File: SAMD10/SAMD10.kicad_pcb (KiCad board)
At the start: 2 copper layers, 18 x 34 mm, 15 parts, among them J0 SWD_PGM, J1 GPIO_A, J2 GPIO_B, J3 Battery, SW1 SW_Push, U1 ATSAMD10C14A-SS, U2 AP7333-33SRG-7

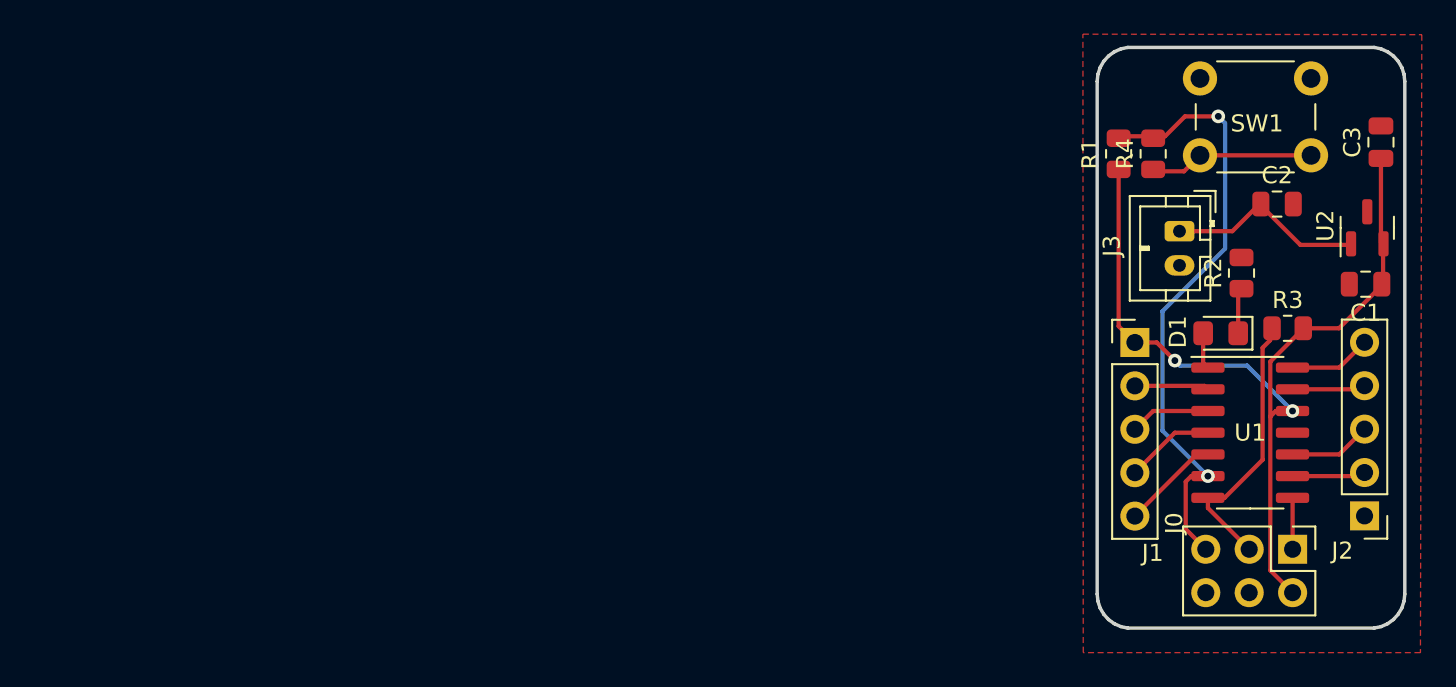
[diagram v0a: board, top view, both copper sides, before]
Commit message: update schematics
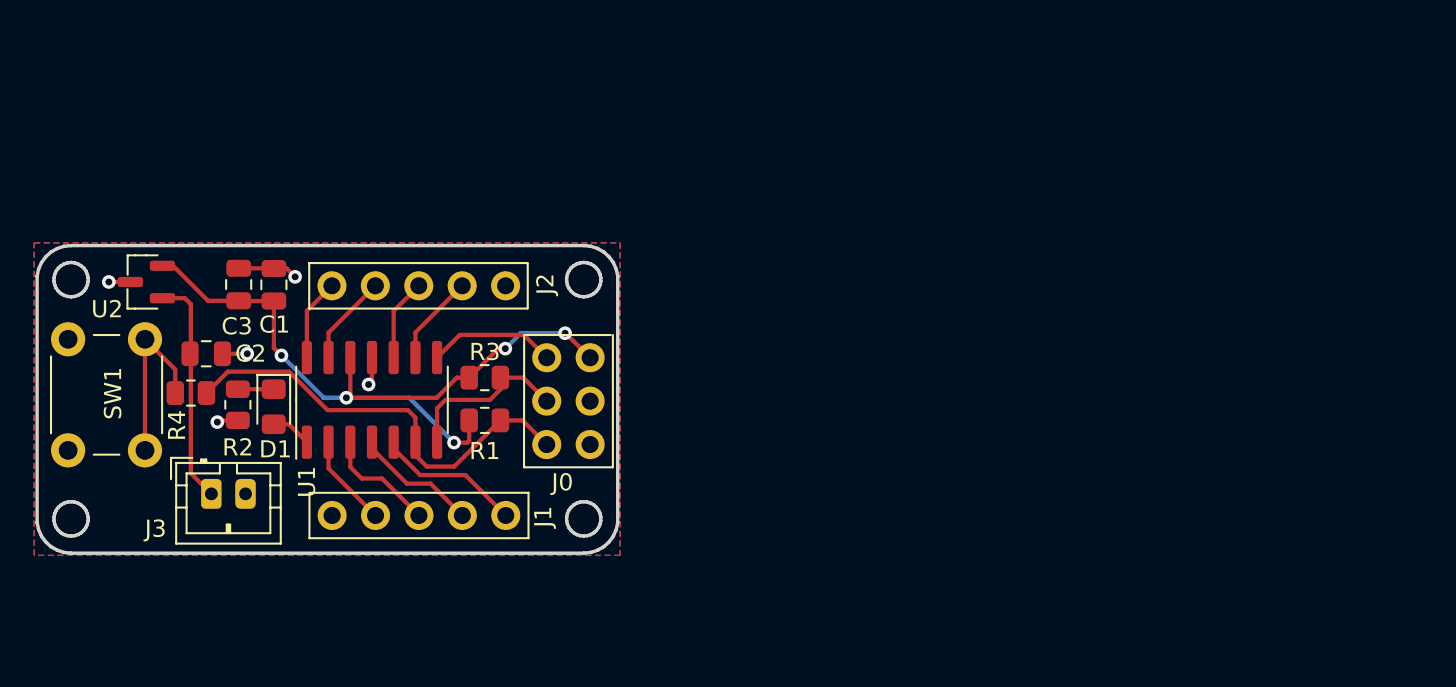
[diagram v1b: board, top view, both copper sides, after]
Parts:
- moved U2 71.5 mm to (135.6, 95.0), turned to 180 degrees
- moved SW1 69.1 mm to (135.5, 98.4), turned to -90 degrees
- moved C3 67.4 mm to (141.0, 95.2)
- moved C1 63.9 mm to (143.1, 95.2), turned to 90 degrees
- moved C2 63.3 mm to (139.1, 99.2)
- moved R2 59.2 mm to (140.9, 102.2), turned to -90 degrees
- moved J3 58.7 mm to (139.4, 107.4), turned to 0 degrees
- moved R4 58.0 mm to (138.2, 101.5), turned to 0 degrees
- moved D1 55.6 mm to (143.1, 102.3), turned to -90 degrees
- moved J2 52.0 mm to (156.6, 95.2), turned to -90 degrees
- moved U1 51.4 mm to (148.8, 101.9), turned to 90 degrees
- moved J1 48.1 mm to (146.5, 108.7), turned to 90 degrees
- moved R3 47.1 mm to (155.4, 100.6), turned to 180 degrees
- moved J0 45.1 mm to (159.0, 99.4), turned to 0 degrees
- moved R1 40.2 mm to (155.4, 103.1), turned to 0 degrees
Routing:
- net RESET: track 36.0 -> 25.7 mm, vias 2 -> 0
- net GND: track 0.00 -> 9.12 mm, vias 0 -> 5
- net +3V3: track 52.6 -> 43.9 mm, vias 2 -> 5
- net SWCLK: track 16.0 -> 10.7 mm
- net SWDIO: track 3.01 -> 7.52 mm
- net GPIO_4: track 5.77 -> 8.55 mm
- net GPIO_3: track 5.24 -> 7.28 mm
- net GPIO_2: track 4.72 -> 6.65 mm
- net +BATT: track 11.7 -> 13.4 mm
- net GPIO_6: track 4.30 -> 5.63 mm
- net GPIO_8: track 4.30 -> 5.63 mm
- net GPIO_1: track 4.36 -> 5.43 mm
- net Net-(R4-Pad1): track 9.63 -> 10.4 mm
- net Net-(D1-Pad1): track 2.70 -> 2.10 mm
- added copper zone on F.Cu, net +3V3
- added copper zone on B.Cu, net GND
- removed copper zone on F.Cu, net GND
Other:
- board size 18 x 34 mm -> 34 x 18 mm
